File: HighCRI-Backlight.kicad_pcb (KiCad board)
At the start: 2 copper layers, 100 x 100 mm, 123 parts, among them J1 Conn_01x03, J2 Screw_Terminal_01x02, J3 Screw_Terminal_01x02, Q1 AOD4130, Q2 AOD4130, Q3 AOD4130, U1 L78L24_SO8, U2 LM324

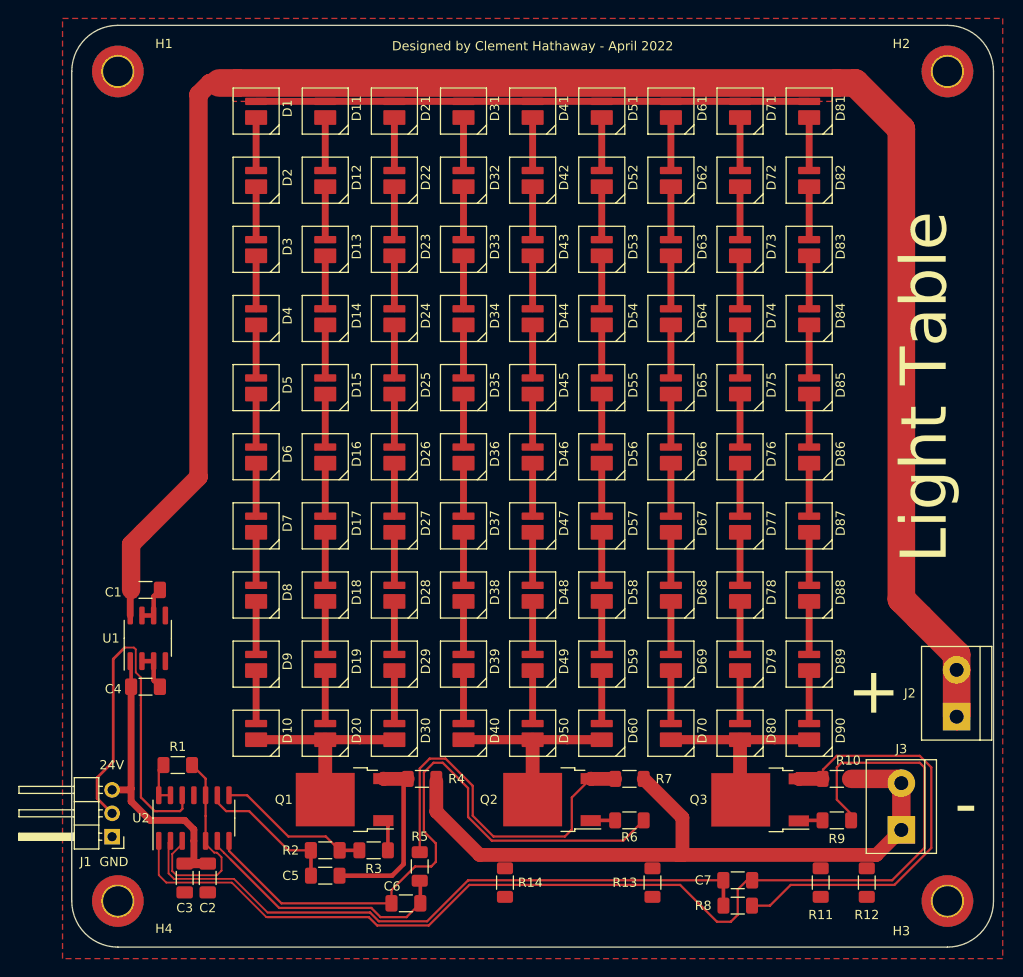
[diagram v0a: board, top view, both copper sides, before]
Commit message: Minor errors
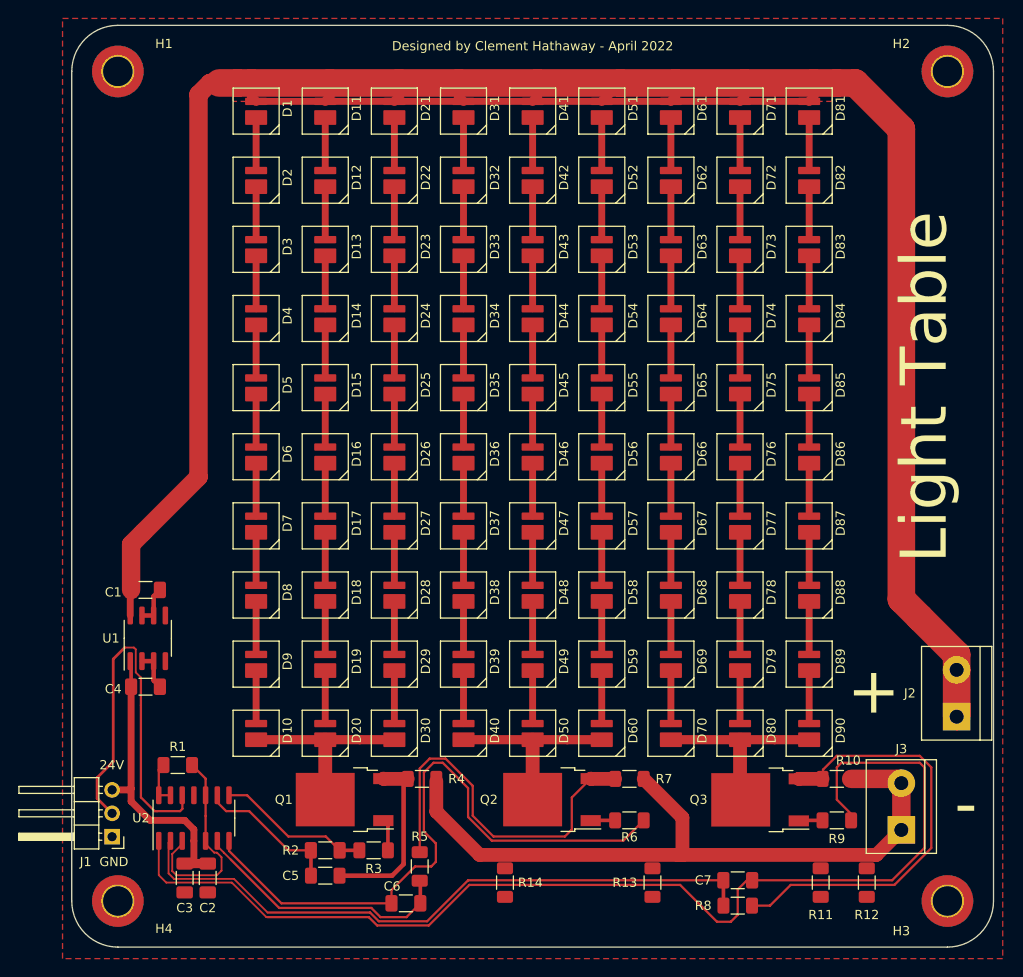
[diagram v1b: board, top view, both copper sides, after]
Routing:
- net +36V: track 264.7 -> 285.2 mm
